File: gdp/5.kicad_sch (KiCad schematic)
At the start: 10 parts, among them IC29 74LS538, IC30 74LS538, IC67 74LS166, IC68 74LS30, IC69 74LS166, IC70 74LS30

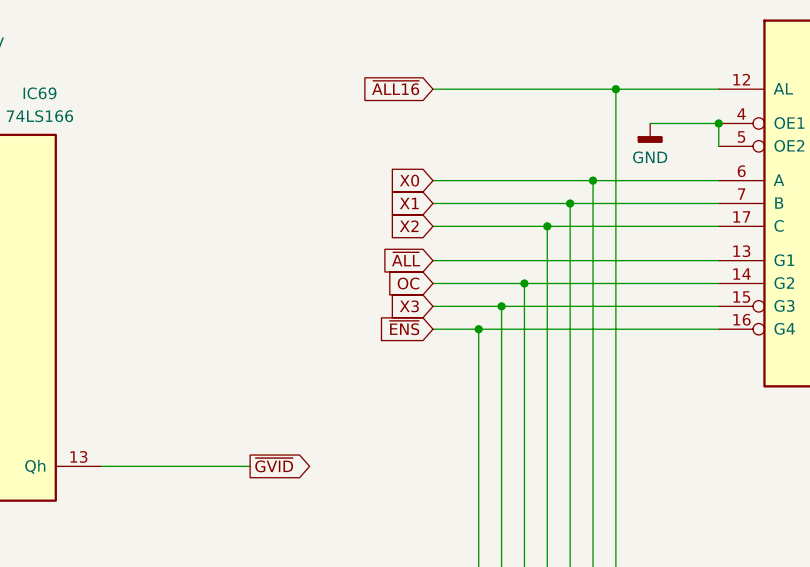
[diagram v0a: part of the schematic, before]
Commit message: Fixes several mistakes (1 mistake in the schema!)
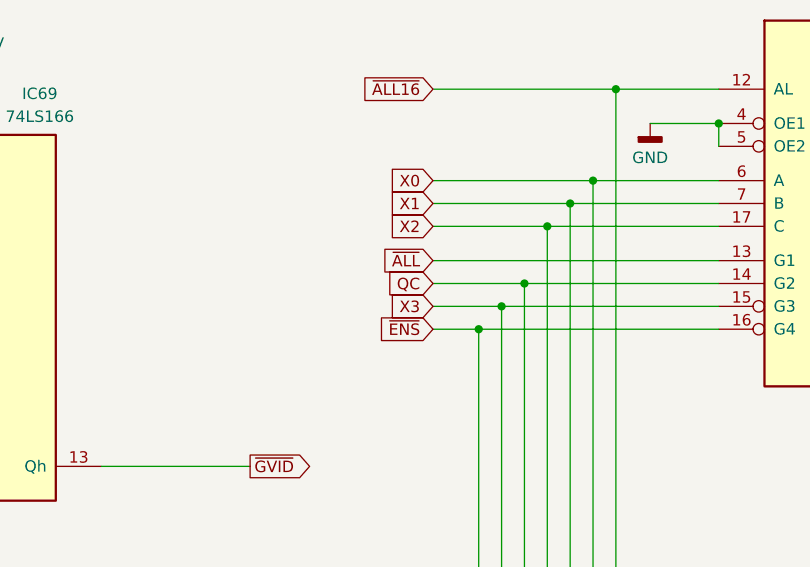
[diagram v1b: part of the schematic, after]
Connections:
- net OC renamed QC
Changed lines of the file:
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@@
 		)
 	)
-	(global_label "OC"
+	(global_label "QC"
 		(shape input)
 		(at 177.8 64.77 180)
